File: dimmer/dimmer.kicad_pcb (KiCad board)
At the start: 2 copper layers, 16 parts, among them J1 Conn_01x04, J2 Conn_01x04, Q1 TIC216, U1 4N25, U2 MOC3021M

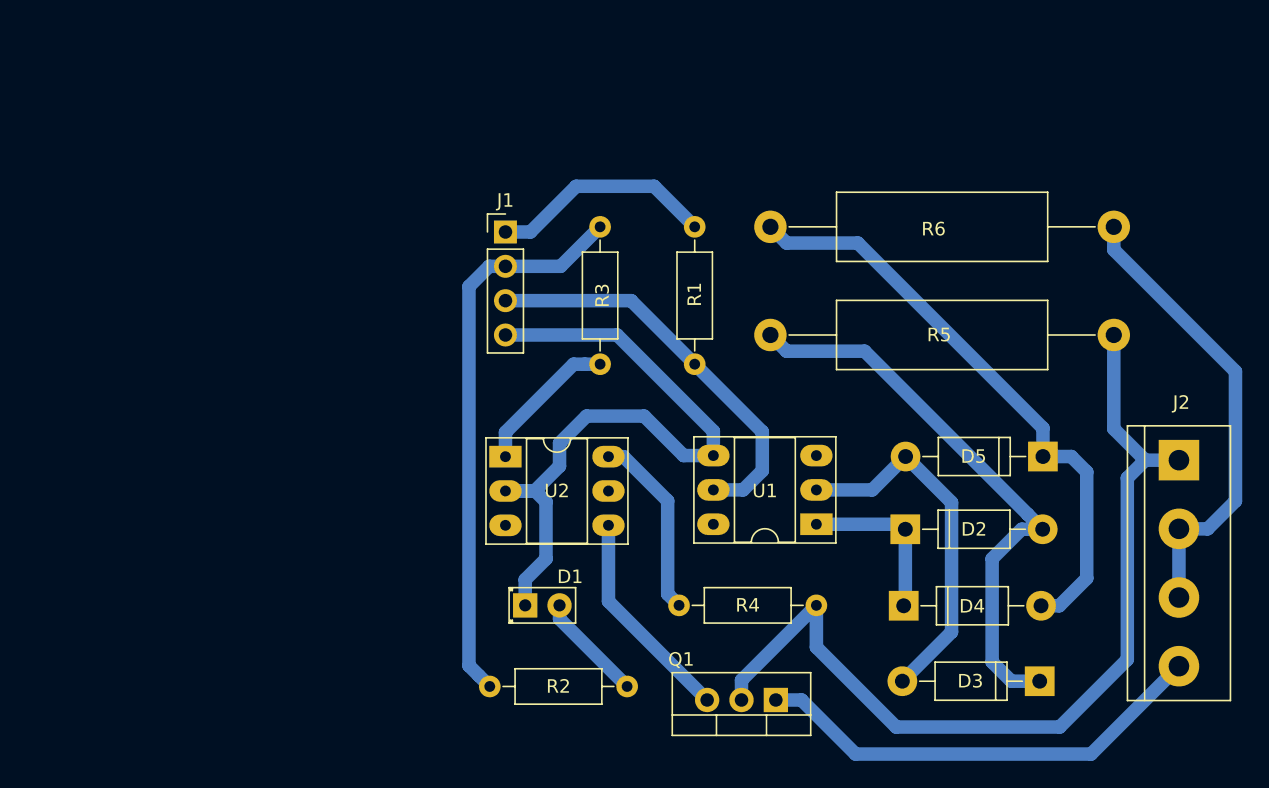
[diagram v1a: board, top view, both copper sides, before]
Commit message: Update dimmer.kicad_pcb
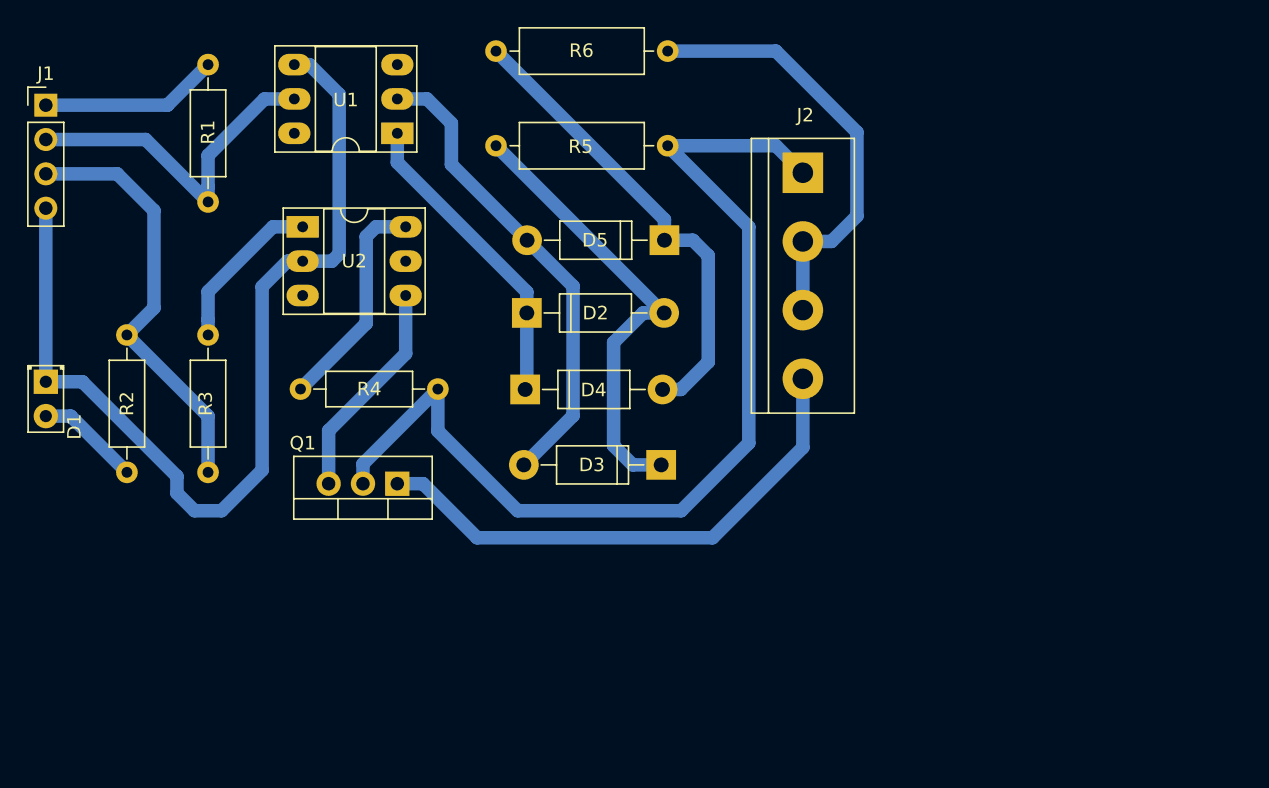
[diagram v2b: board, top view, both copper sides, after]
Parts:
- R5, R6: footprint Resistors_THT:R_Axial_DIN0516_L15.5mm_D5.0mm_P25.40mm_Horizontal -> Resistor_THT:R_Axial_DIN0309_L9.0mm_D3.2mm_P12.70mm_Horizontal
- moved U1 42.4 mm to (148.0, 87.1)
- moved D1 39.1 mm to (122.0, 105.5), turned to 270 degrees
- moved R1 37.9 mm to (134.0, 82.0)
- moved R2 37.4 mm to (128.0, 102.0), turned to 270 degrees
- moved R5 35.8 mm to (168.0, 88.0)
- moved R6 35.5 mm to (168.0, 81.0)
- moved J1 35.3 mm to (122.0, 85.0)
- moved J2 35.0 mm to (178.0, 90.0)
- moved D2 32.2 mm to (157.6, 100.4)
- moved D3 32.2 mm to (167.5, 111.6)
- moved D4 32.2 mm to (157.5, 106.0)
- moved D5 32.2 mm to (167.8, 95.0)
- moved Q1 32.2 mm to (148.0, 113.0)
- moved R4 32.2 mm to (151.0, 106.0)
- moved R3 29.1 mm to (134.0, 102.0), turned to 270 degrees
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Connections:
- J1 pad 2: dimmer -> zero-c
- J1 pad 3: zero-c -> dimmer
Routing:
- net GND: track 51.6 -> 71.1 mm
- net Net-(D2-Pad1): track 12.4 -> 23.0 mm
- net dimmer: track 41.7 -> 31.8 mm
- net Net-(D4-Pad2): track 44.2 -> 35.0 mm
- net Net-(D2-Pad2): track 42.5 -> 34.0 mm
- net Net-(D3-Pad2): track 27.2 -> 35.3 mm
- net VAC: track 67.9 -> 75.2 mm
- net Net-(J2-Pad4): track 34.2 -> 39.5 mm
- net zero-c: track 30.1 -> 25.5 mm
- net VCC: track 16.6 -> 13.2 mm
- net Net-(R4-Pad2): track 13.8 -> 16.5 mm
- net NEUT: track 34.1 -> 32.5 mm
- net Net-(R3-Pad1): track 10.9 -> 12.2 mm
